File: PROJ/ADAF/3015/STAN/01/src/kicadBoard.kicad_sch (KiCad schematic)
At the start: 13 parts

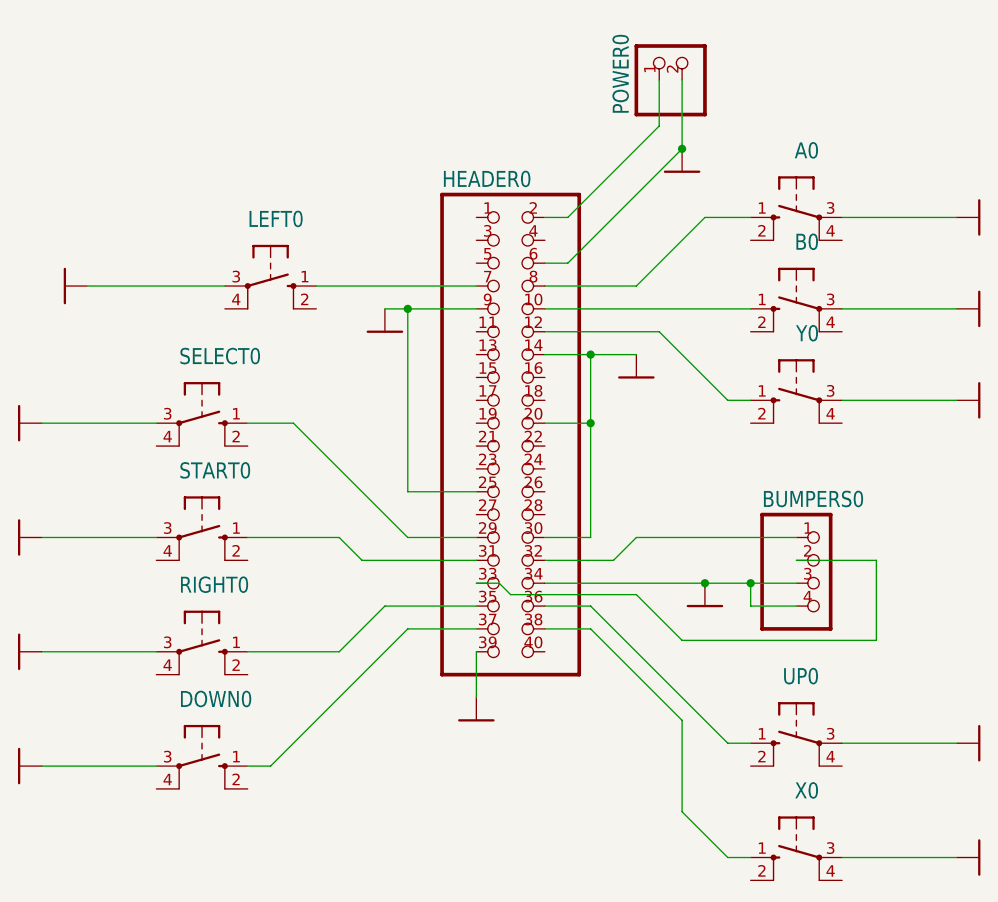
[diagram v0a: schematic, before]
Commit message: Quickly Adding Everything
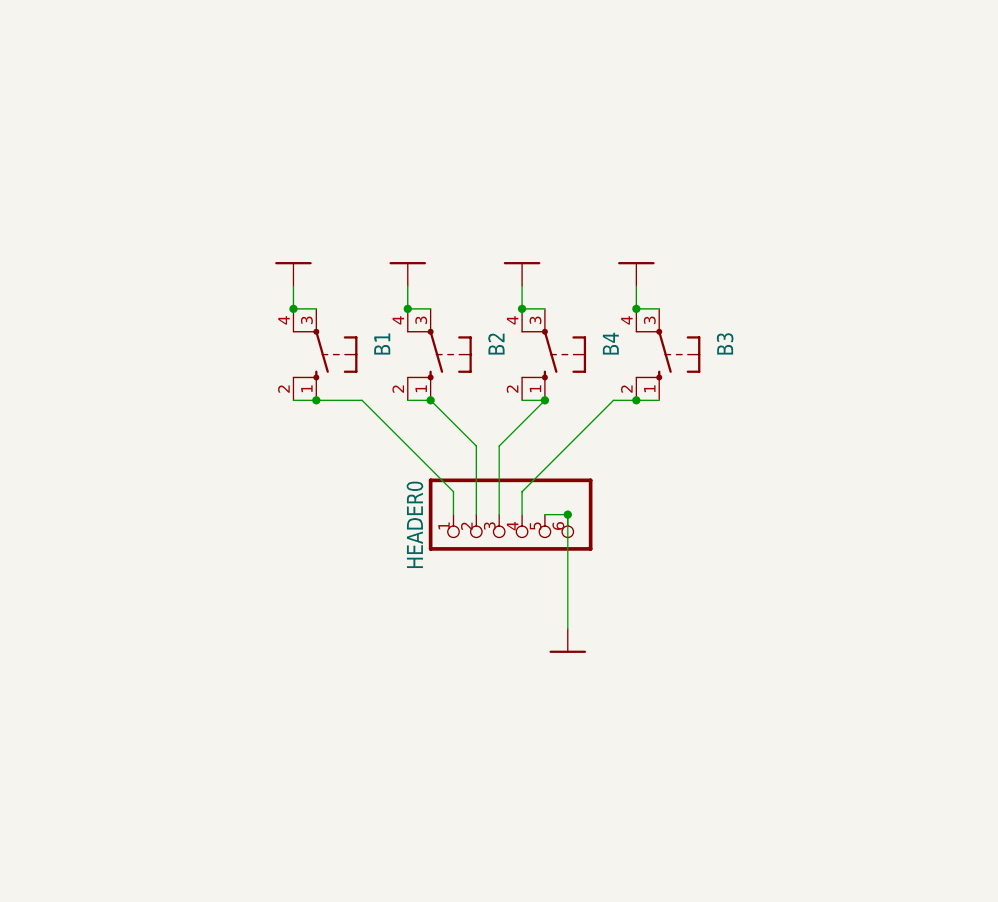
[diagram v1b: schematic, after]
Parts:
- removed A0, B0, DOWN0, LEFT0, RIGHT0, SELECT0, START0, UP0, X0, Y0: (no value), symbol eagleSchem-eagle-import:10-XX
- removed BUMPERS0: (no value), symbol eagleSchem-eagle-import:PINHD-1X4
- removed HEADER0: (no value), symbol eagleSchem-eagle-import:PINHD-2X20
- removed POWER0: (no value), symbol eagleSchem-eagle-import:PINHD-1X2
- added B1, B2, B3, B4: (no value), symbol schematicEagle-eagle-import:10-XX
- added HEADER0: (no value), symbol schematicEagle-eagle-import:PINHD-1X6
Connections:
- net GND: now also B1.3 (P), B1.4 (P1), B2.3 (P), B2.4 (P1), B3.3 (P), B3.4 (P1), B4.3 (P), B4.4 (P1), HEADER0.5, HEADER0.6
- new net: B4.1 (S), B4.2 (S1), HEADER0.3
- new net: B1.1 (S), B1.2 (S1), HEADER0.1
- new net: B2.1 (S), B2.2 (S1), HEADER0.2
- new net: B3.1 (S), B3.2 (S1), HEADER0.4

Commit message: Quickly Adding Everything
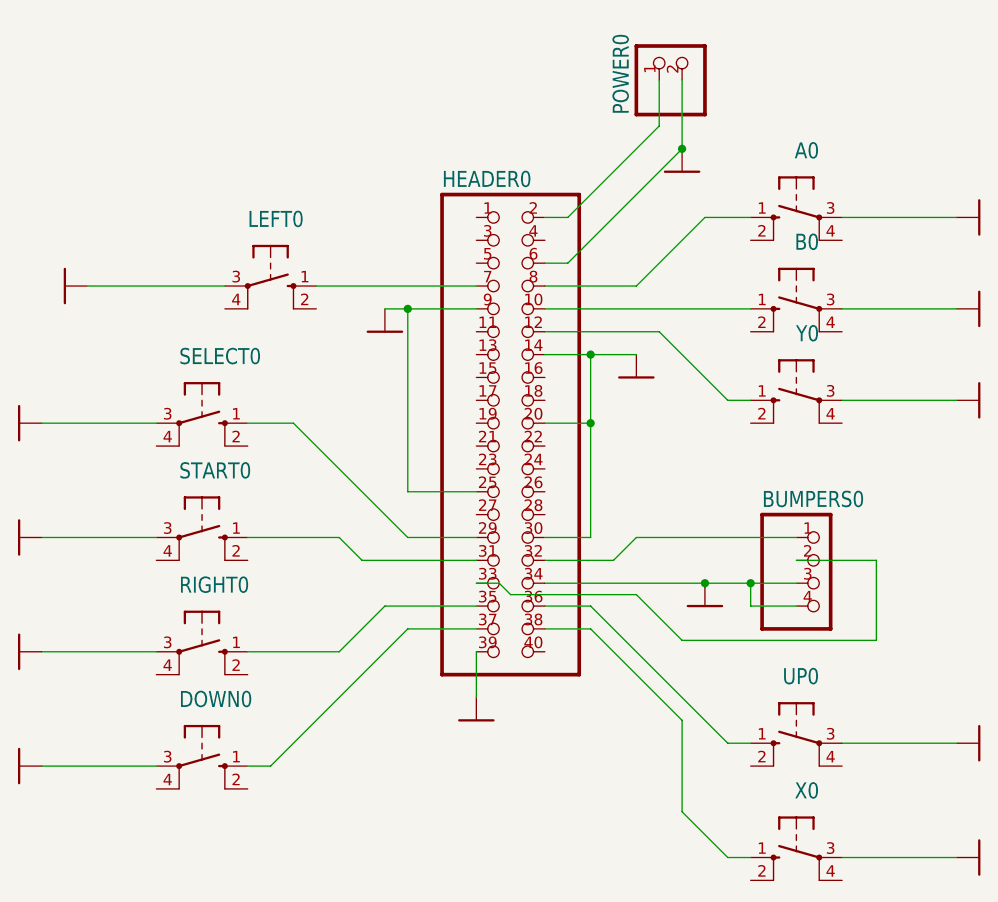
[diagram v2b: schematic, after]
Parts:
- removed B1, B2, B3, B4: (no value), symbol schematicEagle-eagle-import:10-XX
- removed HEADER0: (no value), symbol schematicEagle-eagle-import:PINHD-1X6
- added A0, B0, DOWN0, LEFT0, RIGHT0, SELECT0, START0, UP0, X0, Y0: (no value), symbol eagleSchem-eagle-import:10-XX
- added BUMPERS0: (no value), symbol eagleSchem-eagle-import:PINHD-1X4
- added HEADER0: (no value), symbol eagleSchem-eagle-import:PINHD-2X20
- added POWER0: (no value), symbol eagleSchem-eagle-import:PINHD-1X2
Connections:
- net GND: now also A0.3 (P), B0.3 (P), BUMPERS0.3, BUMPERS0.4, DOWN0.3 (P), HEADER0.14, HEADER0.20, HEADER0.25, HEADER0.30, HEADER0.34, HEADER0.39, HEADER0.6, HEADER0.9, LEFT0.3 (P), POWER0.2, RIGHT0.3 (P), SELECT0.3 (P), START0.3 (P), UP0.3 (P), X0.3 (P), Y0.3 (P)
- new net: HEADER0.36, UP0.1 (S)
- new net: HEADER0.29, SELECT0.1 (S)
- new net: B0.1 (S), HEADER0.10
- new net: HEADER0.12, Y0.1 (S)
- new net: HEADER0.2, POWER0.1
- new net: HEADER0.31, START0.1 (S)
- new net: BUMPERS0.1, HEADER0.32
- new net: BUMPERS0.2, HEADER0.33
- new net: HEADER0.35, RIGHT0.1 (S)
- new net: DOWN0.1 (S), HEADER0.37
- new net: HEADER0.38, X0.1 (S)
- new net: HEADER0.7, LEFT0.1 (S)
- new net: A0.1 (S), HEADER0.8
